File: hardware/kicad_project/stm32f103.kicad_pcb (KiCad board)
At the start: 2 copper layers, 86 x 45 mm, 61 parts, among them J1 SWD, J2 USART1, J3 USB4105-GF-A, J4 Conn_01x30, J5 INA226 ALERT, J6 USB1130-15-A_REVA, M1 Mounting_Holes_3mm_THT, M2 Mounting_Holes_3mm_THT, M3 Mounting_Holes_3mm_THT, M4 Mounting_Holes_3mm_THT, Q1 Q_PNP_BEC, SW1 1825910-6, U1 LM1117-3.3, U2 STM32F103RCTx, U3 INA226AIDGSR, U4 W25Q32JVSS, Y1 8M

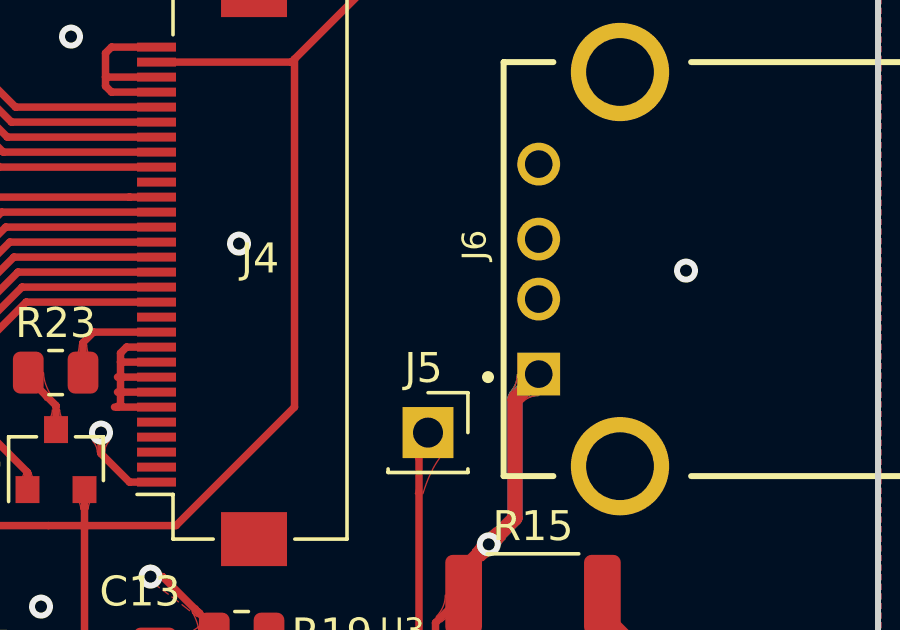
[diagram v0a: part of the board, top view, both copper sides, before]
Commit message: 更新 PCB 工程设置
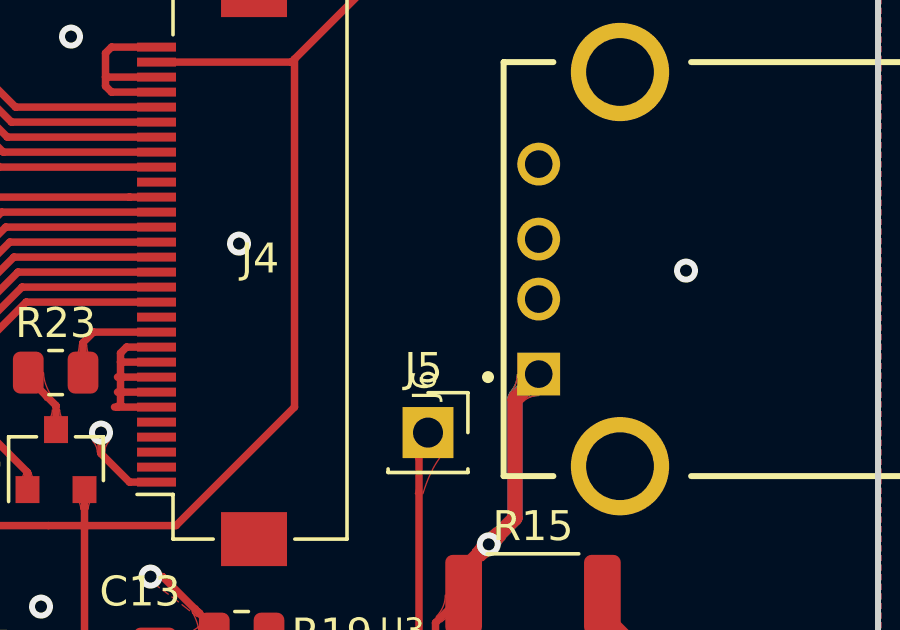
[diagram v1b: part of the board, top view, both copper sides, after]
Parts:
- J3: footprint DL_Usb_C_USB4105-GF-A:DL_Usb_C_USB4105-GF-A -> 3rd_USB4105-GF-A:3rd_USB4105-GF-A(USB-C)
- J6: footprint DL_Usb_A_USB1130-15-A_REVA:DL_Usb_A_USB1130-15-A_REVA -> 3rd_USB1130-15-A_REVA:3rd_USB1130-15-A_REVA(USB-A)
- S1, S2, S3, S4: footprint DL_Key_Hori_B3F-3100:DL_Key_Hori_B3F-3100 -> 3rd_B3F-3100:3rd_B3F-3100(Key_Hori)
- SW1: footprint DL_Key_Vertical_B3F-1000:DL_Key_Vertical_B3F-1000 -> 3rd_B3F-1000:3rd_B3F-1000(Key_Vertical)
- U3: footprint DL_Ina226_INA226AIDGSR:DL_Ina226_SOP50P490X110-10N -> 3rd_INA226AIDGSR:3rd_SOP50P490X110-10N(INA226AIDGSR)
- U4: footprint DL_W25q32_W25Q32JVSSIQ:DL_W25q32_SOIC127P790X216-8N -> 3rd_W25Q32JVSSIQ:3rd_SOIC127P790X216-8N(W25Q32JVSSIQ)
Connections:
- J3 pad A8: Net-(J3-PadA8) -> unconnected-(J3-PadA8)
- J3 pad B8: Net-(J3-PadB8) -> unconnected-(J3-PadB8)
- J4 pad 12: Net-(J4-Pad12) -> unconnected-(J4-Pad12)
- J4 pad 2: Net-(J4-Pad2) -> unconnected-(J4-Pad2)
- J4 pad 21: Net-(J4-Pad21) -> unconnected-(J4-Pad21)
- J4 pad 3: Net-(J4-Pad3) -> unconnected-(J4-Pad3)
- J4 pad 4: Net-(J4-Pad4) -> unconnected-(J4-Pad4)
- J4 pad 5: Net-(J4-Pad5) -> unconnected-(J4-Pad5)
- J6 pad 2: Net-(J6-Pad2) -> unconnected-(J6-Pad2)
- J6 pad 3: Net-(J6-Pad3) -> unconnected-(J6-Pad3)
- U2 pad 10: Net-(U2-Pad10) -> unconnected-(U2-Pad10)
- U2 pad 11: Net-(U2-Pad11) -> unconnected-(U2-Pad11)
- U2 pad 14: Net-(U2-Pad14) -> unconnected-(U2-Pad14)
- U2 pad 17: Net-(U2-Pad17) -> unconnected-(U2-Pad17)
- U2 pad 20: Net-(U2-Pad20) -> unconnected-(U2-Pad20)
- U2 pad 27: Net-(U2-Pad27) -> unconnected-(U2-Pad27)
- U2 pad 29: Net-(U2-Pad29) -> unconnected-(U2-Pad29)
- U2 pad 30: Net-(U2-Pad30) -> unconnected-(U2-Pad30)
- U2 pad 4: Net-(U2-Pad4) -> unconnected-(U2-Pad4)
- U2 pad 50: Net-(U2-Pad50) -> unconnected-(U2-Pad50)
- U2 pad 55: Net-(U2-Pad55) -> unconnected-(U2-Pad55)
- U2 pad 56: Net-(U2-Pad56) -> unconnected-(U2-Pad56)
- U2 pad 61: Net-(U2-Pad61) -> unconnected-(U2-Pad61)
- U2 pad 62: Net-(U2-Pad62) -> unconnected-(U2-Pad62)
- U2 pad 8: Net-(U2-Pad8) -> unconnected-(U2-Pad8)
- U2 pad 9: Net-(U2-Pad9) -> unconnected-(U2-Pad9)
